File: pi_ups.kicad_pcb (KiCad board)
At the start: 2 copper layers, 92.7 x 53.3 mm, 25 parts, among them J1 Screw_Terminal_01x02, J2 Screw_Terminal_01x02, J3 Conn_02x03_Odd_Even, U1 MCP3428, U2 AP63205WU

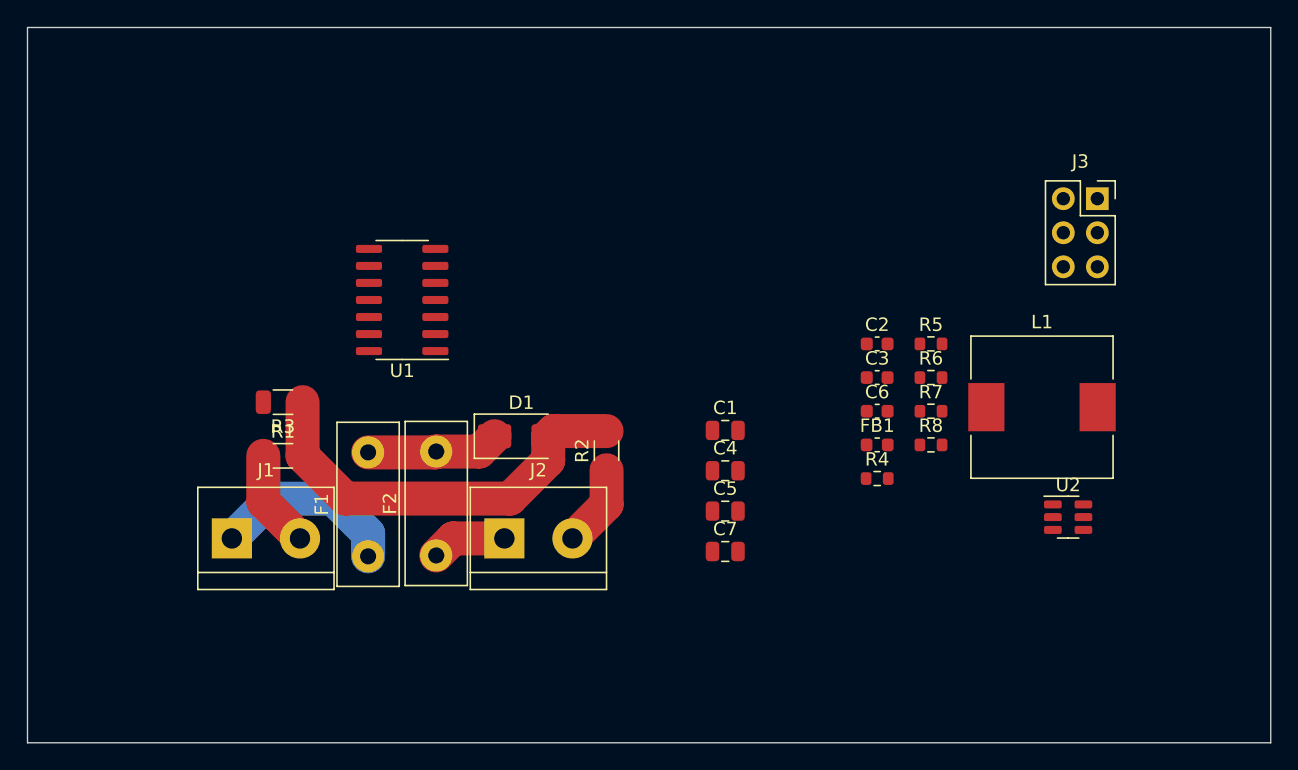
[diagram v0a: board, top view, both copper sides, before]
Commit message: r0.1 board is complete
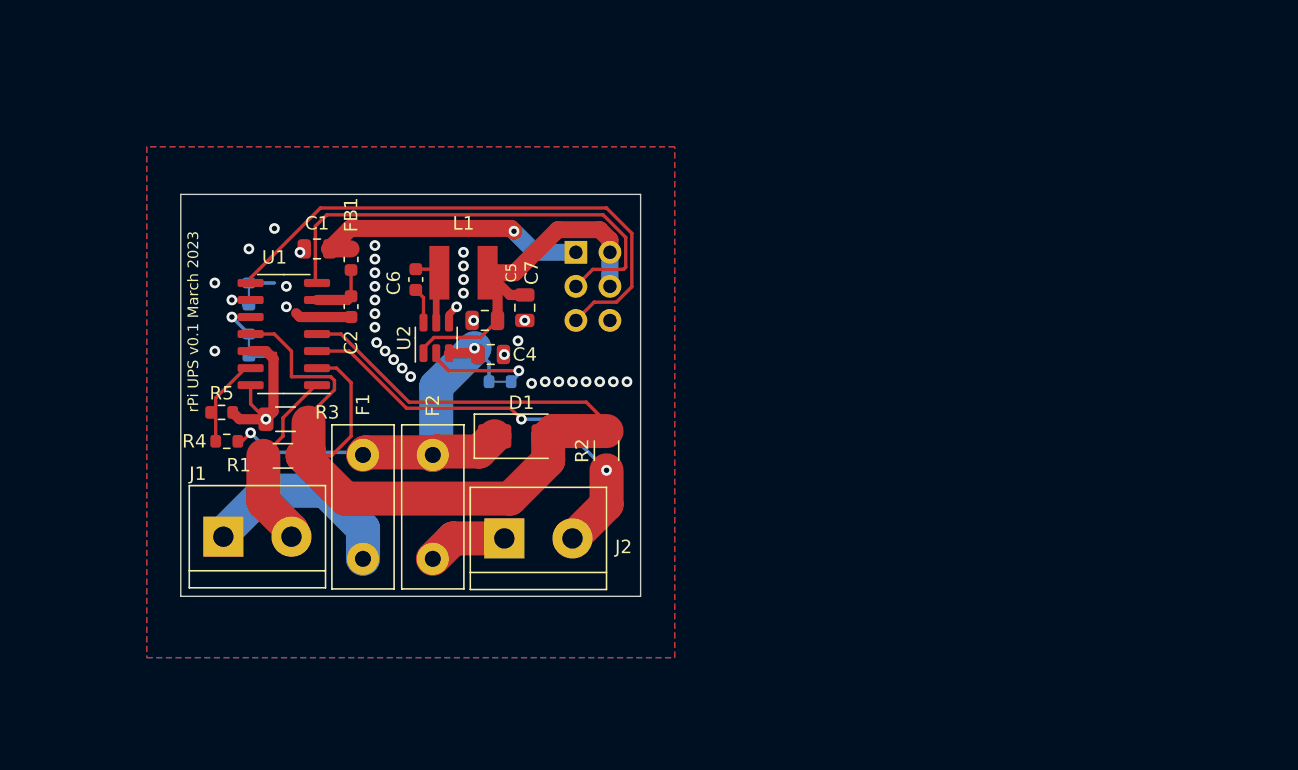
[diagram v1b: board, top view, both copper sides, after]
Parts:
- removed C3: 0.1u, Capacitor_SMD:C_0603_1608Metric
- removed R8: 100k, Resistor_SMD:R_0603_1608Metric
- added JP1: Jumper_2_Bridged, pi_ups:jumper_bridged_0603, B.Cu at (103.8, 97.5)
- ADR0: renamed from R7; value 0 -> Jumper_2_Bridged; footprint Resistor_SMD:R_0603_1608Metric -> pi_ups:jumper_bridged_0603; moved to B.Cu
- ADR1: renamed from R6; value 0 -> Jumper_2_Bridged; footprint Resistor_SMD:R_0603_1608Metric -> pi_ups:jumper_bridged_0603; moved to B.Cu
- J3: moved to B.Cu
- L1: footprint Inductor_SMD:L_10.4x10.4_H4.8 -> pi_ups:NRS5030
- R1, R2, R3: value 10m -> 50m
- R4: value 400k -> 1M
- moved R5 53.1 mm to (83.1, 99.8)
- moved ADR0 51.6 mm to (85.1, 91.0), turned to 90 degrees
- moved ADR1 50.9 mm to (85.1, 94.8), turned to -90 degrees
- moved U2 49.0 mm to (99.1, 94.3), turned to 90 degrees
- moved R4 48.6 mm to (83.4, 102.0), turned to 180 degrees
- moved L1 44.3 mm to (101.1, 89.4)
- moved FB1 41.6 mm to (92.7, 88.4), turned to -90 degrees
- moved C2 39.3 mm to (92.7, 91.9), turned to -90 degrees
- moved J3 39.1 mm to (109.5, 87.9), turned to 180 degrees
- moved C6 35.8 mm to (97.5, 89.9), turned to -90 degrees
- moved C1 33.3 mm to (90.2, 87.6), turned to 180 degrees
- moved C7 23.5 mm to (105.7, 92.0), turned to 90 degrees
- moved C5 22.9 mm to (102.7, 93.0)
- moved C4 19.5 mm to (103.1, 95.5)
- moved U1 9.18 mm to (87.7, 94.0)
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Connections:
- ADR0 pad 1: Net-(U1-Adr1) -> Net-(ADR0-A)
- ADR1 pad 1: Net-(U1-Adr0) -> Net-(ADR1-A)
- U1 pad 10: Net-(U1-Adr1) -> Net-(ADR1-A)
- U1 pad 9: Net-(U1-Adr0) -> Net-(ADR0-A)
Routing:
- net /GNDB: track 31.1 -> 78.6 mm
- net /SCL: track 0.00 -> 40.9 mm
- net /SDA: track 0.00 -> 35.0 mm
- net +5V: track 0.00 -> 28.3 mm
- net VCC: track 9.93 -> 35.8 mm, vias 0 -> 2
- net /Bat2_i: track 6.13 -> 31.4 mm, vias 0 -> 2
- net GND: track 0.00 -> 23.9 mm, vias 0 -> 37
- net +3.3V: track 0.00 -> 21.3 mm, vias 0 -> 1
- net Net-(JP1-A): track 0.00 -> 7.59 mm, vias 0 -> 1
- net /Bat_v: track 0.00 -> 6.76 mm
- net /Bat1_i: track 7.29 -> 13.9 mm
- net Net-(U2-SW): track 0.00 -> 5.68 mm
- net Net-(U1-VDD): track 0.00 -> 4.61 mm
- net Net-(ADR1-A): track 0.00 -> 2.79 mm, vias 0 -> 1
- net Net-(U2-BST): track 0.00 -> 2.68 mm
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- added copper zone on B.Cu, net GND
- added copper zone on F.Cu, net GND
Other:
- board size 92.7 x 53.3 mm -> 34.3 x 30 mm
- board text added: "https://github.com/kamocat/pi_ups"
- board text added: "rPi UPS v0.1 March 2023"
